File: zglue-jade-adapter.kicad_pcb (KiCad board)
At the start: 6 copper layers, 25 x 20 mm, 76 parts, among them J1 543630489, J2 543630489, U1 zGlue-Jade

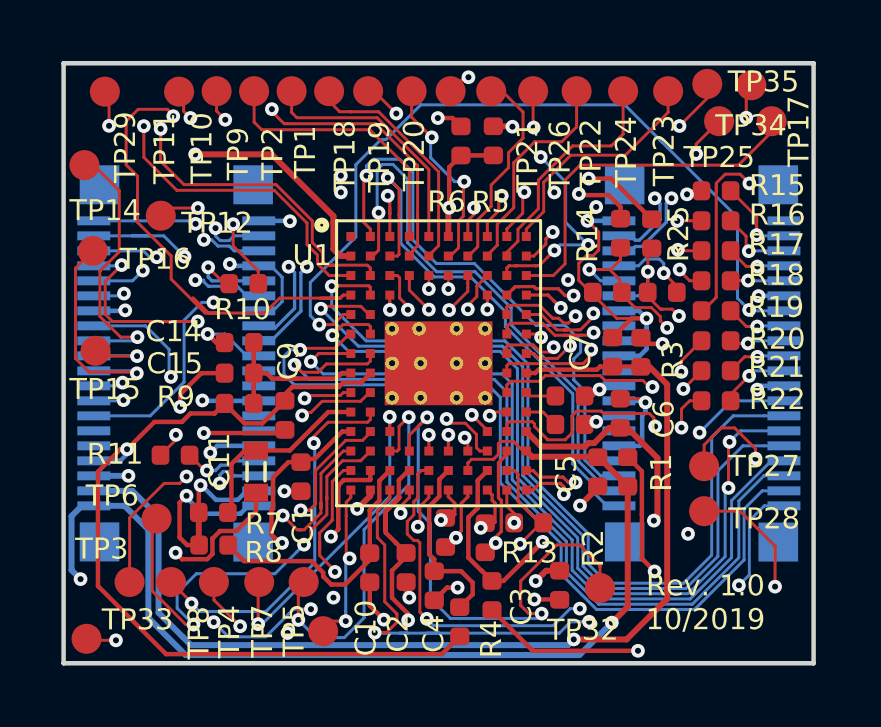
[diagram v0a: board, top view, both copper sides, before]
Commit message: Tune differential pairs
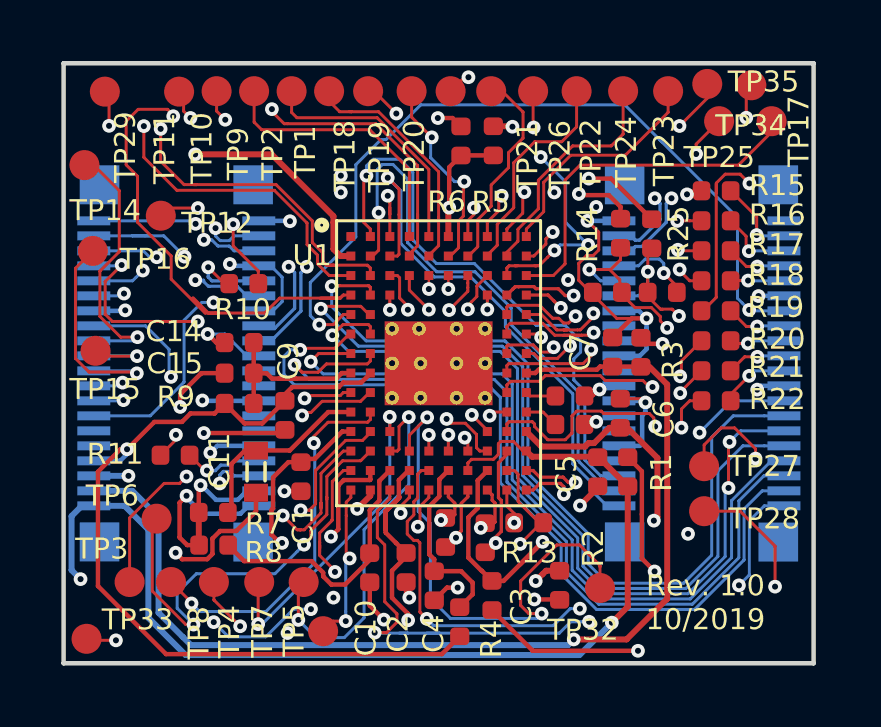
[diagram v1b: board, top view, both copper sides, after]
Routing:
- net /C_CSI_D1_OUT_N: track 10.2 -> 13.7 mm
- net /C_CSI_D1_OUT_P: track 11.0 -> 13.5 mm
- net /PROC_SO: track 22.8 -> 23.4 mm
- net /PROC_SI: track 25.6 -> 26.2 mm
